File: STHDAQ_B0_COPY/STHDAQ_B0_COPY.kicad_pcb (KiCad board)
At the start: 2 copper layers, 33.8 x 56.5 mm, 49 parts, among them J1 532611071, J2 532611071, U1 ADS1256IDBR, U2 ADP151AUJZ-3.0-R7, U3 OPA350UA, U4 REF5025AIDR, U5 INA821IDR, U6 INA821IDR, U7 INA821IDR, U8 INA821IDR, Y1 ABLS-8MHZ-K4T

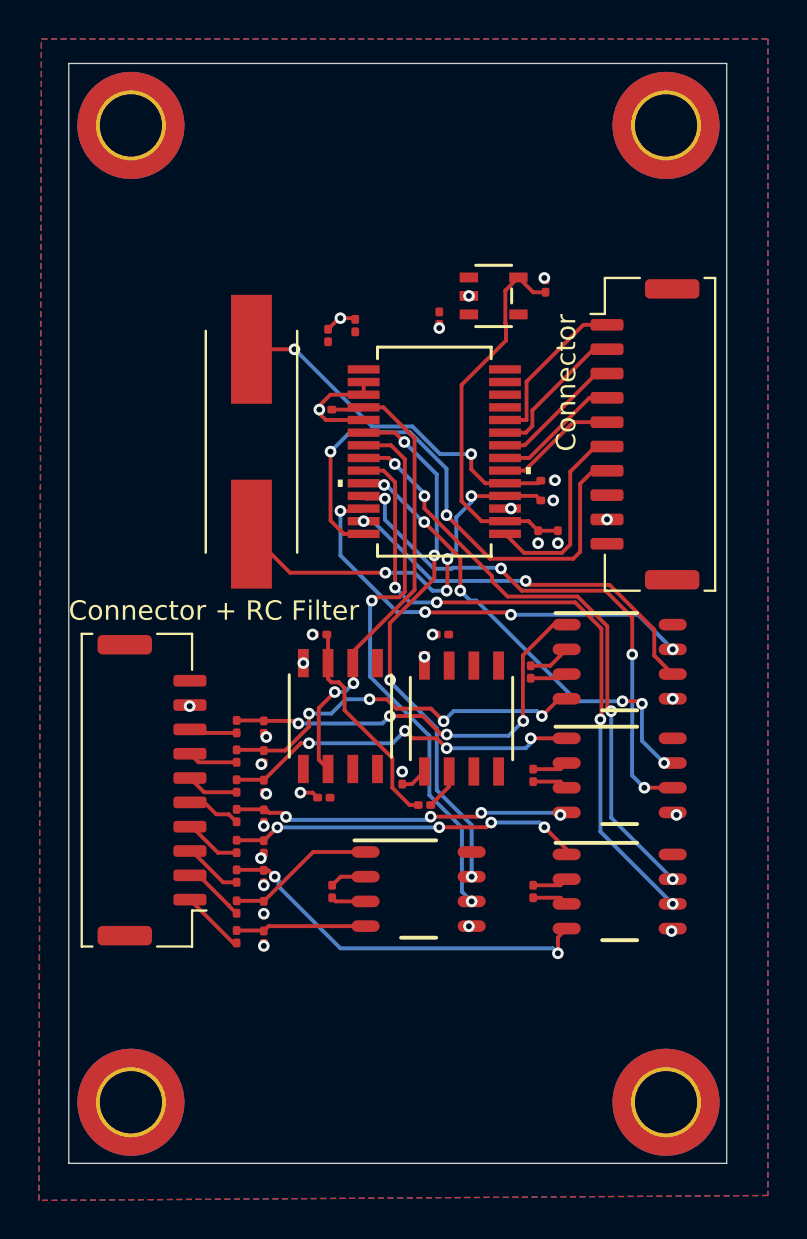
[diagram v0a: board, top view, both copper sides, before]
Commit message: B0 pcb layouting
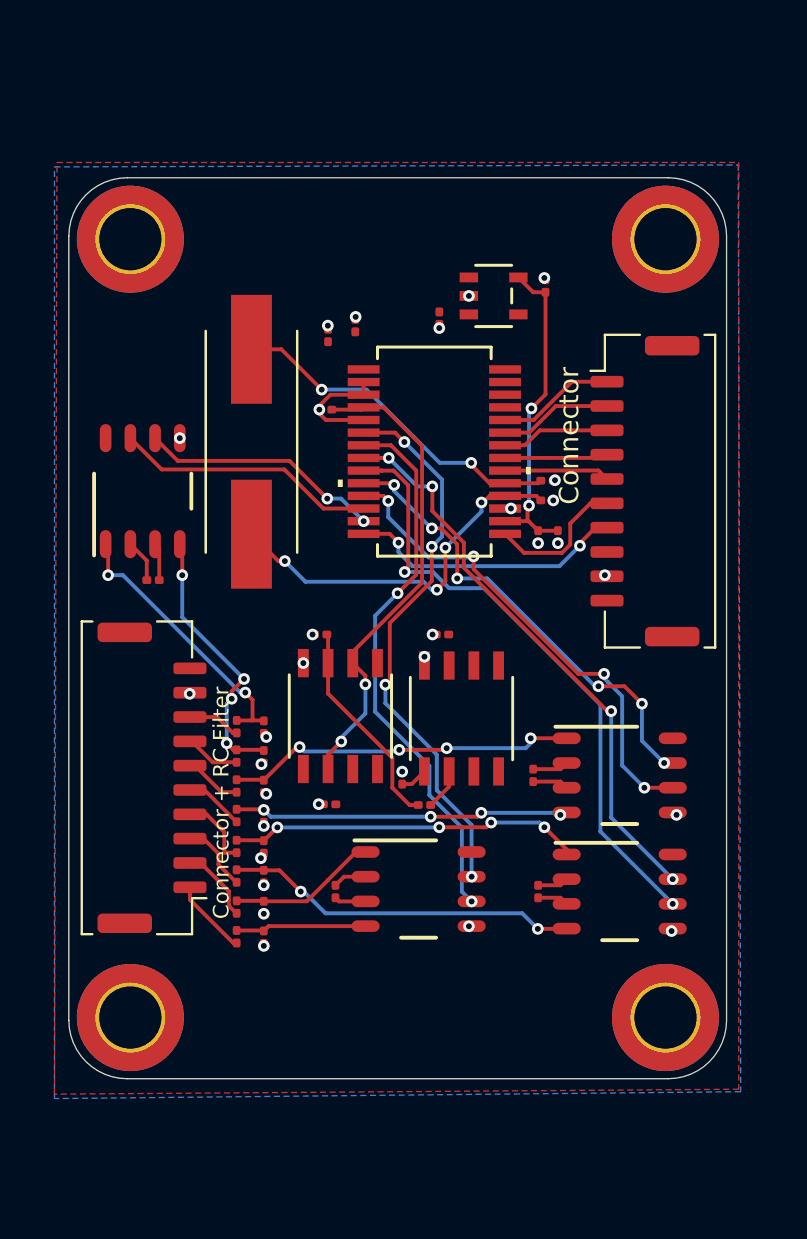
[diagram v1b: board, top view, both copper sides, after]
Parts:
- moved H4 45.8 mm to (183.3, 100.5)
- moved H2 44.4 mm to (183.3, 60.5)
- moved U8 26.0 mm to (183.9, 73.4), turned to 90 degrees
- moved R13 20.0 mm to (184.4, 78.0), turned to 180 degrees
- moved H3 5.85 mm to (210.8, 60.5)
- moved H1 4.35 mm to (210.8, 100.5)
- moved J2 2.92 mm to (209.7, 73.4)
- moved J1 0.63 mm to (184.4, 88.1)
- moved C7 0.46 mm to (193.5, 89.5)
- moved R11 0.25 mm to (204.2, 94.0)
- moved R2 0.17 mm to (193.8, 94.0)
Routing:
- net /SYNC/PDWN: track 28.2 -> 14.4 mm
- net AIN6: track 22.6 -> 13.7 mm, vias 4 -> 0
- net AIN7: track 20.5 -> 12.5 mm
- net /S4-: track 22.0 -> 14.2 mm, vias 4 -> 2
- net /S4+: track 19.6 -> 14.0 mm
- net REF3.3: track 20.0 -> 16.8 mm, vias 0 -> 2
- net /RESET: track 10.1 -> 7.33 mm
- net AIN3: track 34.5 -> 31.8 mm, vias 4 -> 2
- net Earth: track 8.62 -> 6.06 mm, vias 30 -> 31
- net /SCLK: track 8.42 -> 6.06 mm
- net AIN5: track 27.6 -> 25.2 mm
- net /S2+: track 19.9 -> 18.2 mm
- net /DIN: track 7.49 -> 5.81 mm
- net AIN2: track 31.1 -> 29.6 mm
- net /DOUT: track 6.77 -> 5.56 mm
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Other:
- board size 33.8 x 56.5 mm -> 33.8 x 46.3 mm
